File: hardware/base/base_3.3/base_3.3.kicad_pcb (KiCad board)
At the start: 2 copper layers, 69.7 x 17 mm, 8 parts, among them IC1 single_pad, IC2 single_pad, J1 conn_2x2

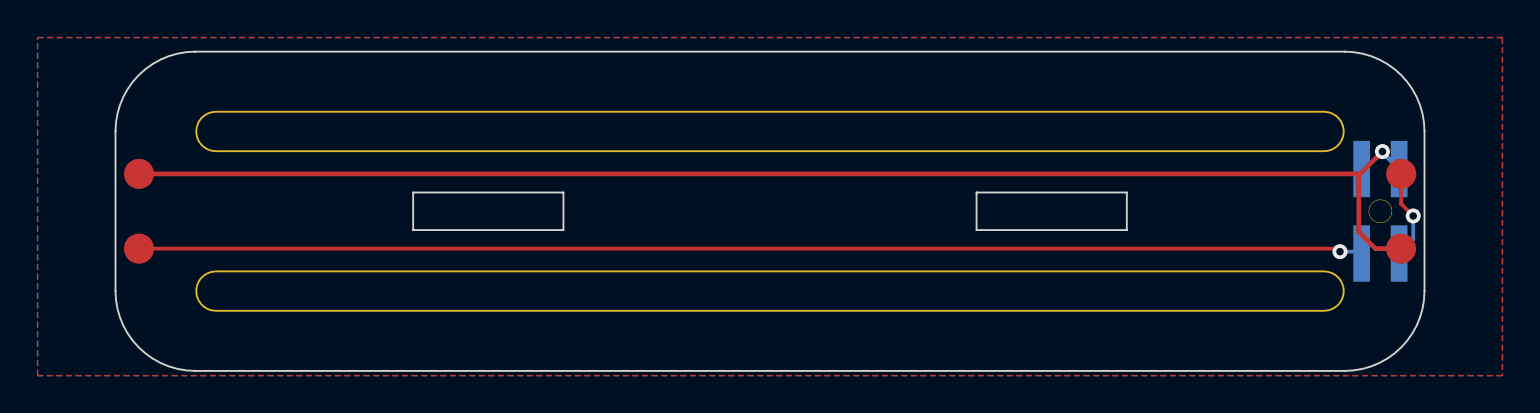
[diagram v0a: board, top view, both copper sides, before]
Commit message: WIP
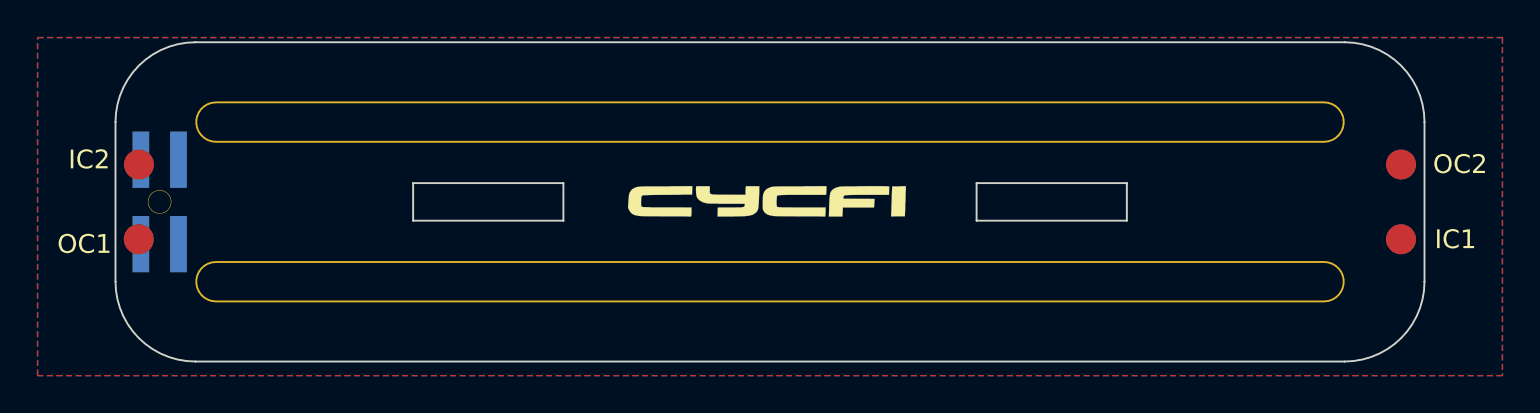
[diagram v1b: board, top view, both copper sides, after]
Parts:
- G***: moved to F.Cu
- moved IC2 67.3 mm to (91.4, 52.8), turned to 0 degrees
- moved OC2 67.3 mm to (158.6, 52.8), turned to 0 degrees
- moved OC1 67.3 mm to (91.4, 56.7), turned to 0 degrees
- moved IC1 67.3 mm to (158.6, 56.7), turned to 0 degrees
- moved J1 65.0 mm to (92.5, 54.8), turned to -90 degrees
- moved H6 9.00 mm to (125.0, 50.5), turned to 180 degrees
- moved H5 8.00 mm to (125.0, 59.0), turned to 180 degrees
- moved G*** 0.71 mm to (124.8, 54.8), turned to 0 degrees
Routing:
- net inner_coil: track 73.7 -> 0.00 mm, vias 1 -> 0
- net /out-: track 65.2 -> 0.00 mm, vias 1 -> 0
- net /out+: track 4.82 -> 0.00 mm, vias 1 -> 0
